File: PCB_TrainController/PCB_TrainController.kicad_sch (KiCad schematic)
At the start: 5 parts, among them J7 Conn_01x10_Socket

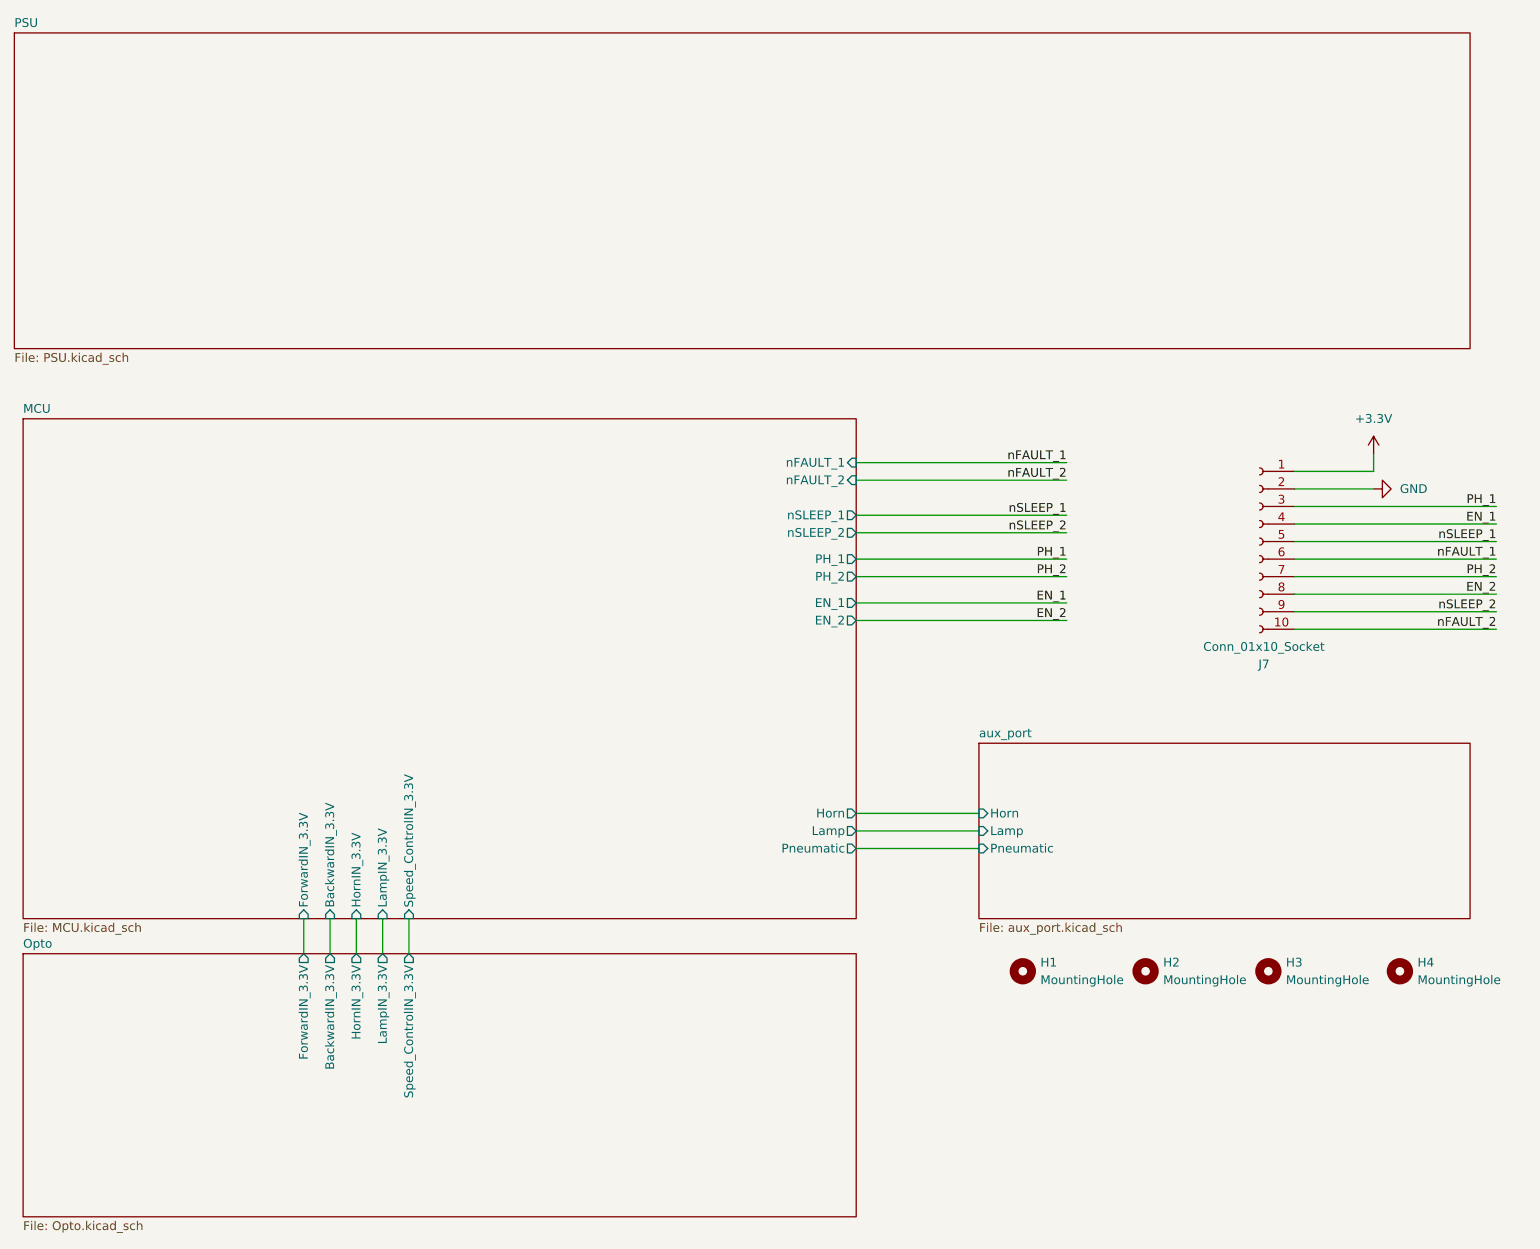
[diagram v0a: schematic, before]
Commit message: Finished
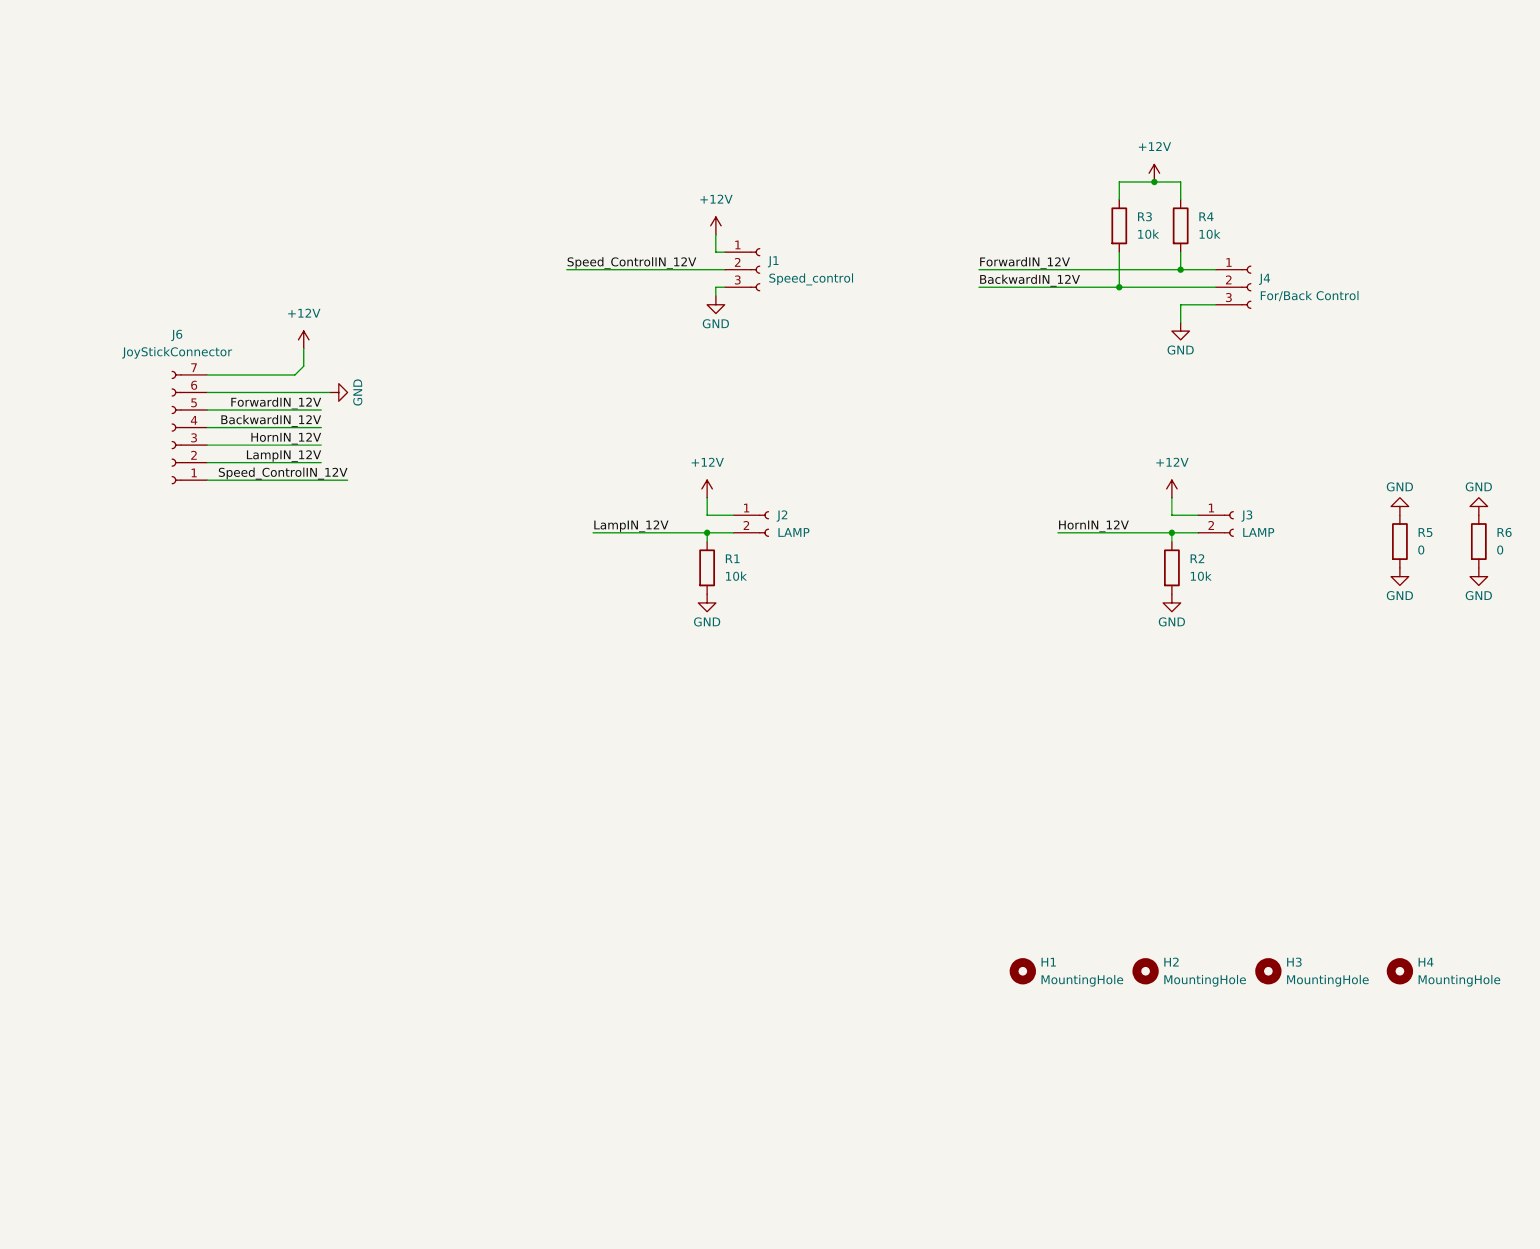
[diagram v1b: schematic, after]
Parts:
- removed J7: Conn_01x10_Socket, Connector_JST:JST_XH_B10B-XH-A_1x10_P2.50mm_Vertical, symbol Connector:Conn_01x10_Socket
- added J1: Speed_control, Connector_JST:JST_XH_B3B-XH-A_1x03_P2.50mm_Vertical, symbol Connector:Conn_01x03_Socket
- added J2, J3: LAMP, Connector_JST:JST_XH_B2B-XH-A_1x02_P2.50mm_Vertical, symbol Connector:Conn_01x02_Socket
- added J4: For/Back Control, Connector_JST:JST_XH_B3B-XH-A_1x03_P2.50mm_Vertical, symbol Connector:Conn_01x03_Socket
- added J6: JoyStickConnector, Connector_JST:JST_XH_S7B-XH-A_1x07_P2.50mm_Horizontal, symbol Connector:Conn_01x07_Socket
- added R1, R2, R3, R4: 10k, Resistor_SMD:R_0805_2012Metric, symbol Device:R
- added R5, R6: 0, Resistor_THT:R_Axial_DIN0204_L3.6mm_D1.6mm_P5.08mm_Horizontal, symbol Device:R
- H1, H2, H3, H4: footprint MountingHole:MountingHole_5.3mm_M5_DIN965_Pad -> MountingHole:MountingHole_3.2mm_M3_DIN965_Pad_TopBottom
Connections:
- net GND: now also J1.3 (Pin_3), J4.3 (Pin_3), J6.6 (Pin_6), R1.2, R2.2, R5.1, R5.2, R6.1, R6.2
- new net +12V: J1.1 (Pin_1), J2.1 (Pin_1), J3.1 (Pin_1), J6.7 (Pin_7), R3.1, R4.1
- new net BackwardIN_12V: J4.2 (Pin_2), J6.4 (Pin_4), R3.2
- new net ForwardIN_12V: J4.1 (Pin_1), J6.5 (Pin_5), R4.2
- new net HornIN_12V: J3.2 (Pin_2), J6.3 (Pin_3), R2.1
- new net LampIN_12V: J2.2 (Pin_2), J6.2 (Pin_2), R1.1
- new net Speed_ControlIN_12V: J1.2 (Pin_2), J6.1 (Pin_1)
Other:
- removed sheet MCU
- removed sheet Opto
- removed sheet PSU
- removed sheet aux_port
